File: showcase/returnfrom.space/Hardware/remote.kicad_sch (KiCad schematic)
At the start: 3 parts, among them J7 OLED, U6 ESP32-S2-SOLO

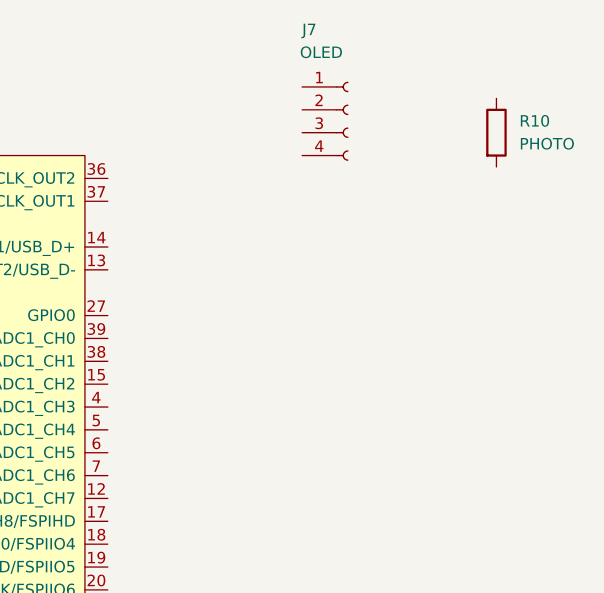
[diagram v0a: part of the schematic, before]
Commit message: updated
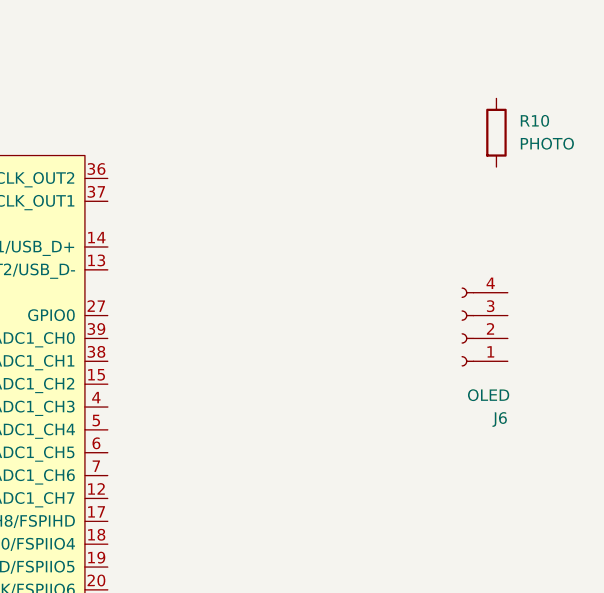
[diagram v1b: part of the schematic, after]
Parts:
- removed J7: OLED, Connector_PinSocket_2.54mm:PinSocket_1x04_P2.54mm_Vertical, symbol Connector:Conn_01x04_Socket
- added J6: OLED, TG9541:Display_128x64_096_I2C, symbol Connector:Conn_01x04_Socket
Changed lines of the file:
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@@
 	(paper "A4")
+	(symbol
+		(lib_id "Connector:Conn_01x04_Socket")
+		(at 173.99 62.23 180)
+		(unit 1)
+		(exclude_from_sim no)
+		(in_bom yes)
+		(on_board yes)
+		(dnp no)
+		(property "Reference" "J6"
+			(at 179.07 71.12 0)
+			(effects
+				(font
+					(size 1.27 1.27)
+				)
+				(justify left)
+			)
+		)
+		(property "Value" "OLED"
+			(at 179.324 68.58 0)
+			(effects
+				(font
+					(size 1.27 1.27)
+				)
+				(justify left)
+			)
+		)
+		(property "Footprint" "TG9541:Display_128x64_096_I2C"
+			(at 173.99 62.23 0)
+			(effects
+				(font
+					(size 1.27 1.27)
+				)
+				(hide yes)
+			)
+		)
+		(property "Datasheet" "~"
+			(at 173.99 62.23 0)
+			(effects
+				(font
+					(size 1.27 1.27)
+				)
+				(hide yes)
+			)
+		)
+		(property "Description" "Generic connector, single row, 01x04, script generated"
+			(at 173.99 62.23 0)
+			(effects
+				(font
+					(size 1.27 1.27)
+				)
+				(hide yes)
+			)
+		)
+		(pin "4"
+		)
+		(pin "3"
+		)
+		(pin "2"
+		)
+		(pin "1"
+		)
+		(instances
+			(project "spacescape"
+				(path "/418a52ba-b136-48f0-a485-149e9dc1363e/bd4ffa4f-b637-4be7-8de2-092b7a28716e"
+					(reference "J6")
+					(unit 1)
+				)
+			)
+		)
+	)
 	(symbol
 		(lib_id "Device:R")
@@
 					(unit 1)
 				)
-			)
-		)
-	)
-	(symbol
-		(lib_id "Connector:Conn_01x04_Socket")
-		(at 161.29 36.83 0)
-		(unit 1)
-		(exclude_from_sim no)
-		(in_bom yes)
-		(on_board yes)
-		(dnp no)
-		(property "Reference" "J7"
-			(at 156.21 27.94 0)
-			(effects
-				(font
-					(size 1.27 1.27)
-				)
-				(justify left)
-			)
-		)
-		(property "Value" "OLED"
-			(at 155.956 30.48 0)
-			(effects
-				(font
-					(size 1.27 1.27)
-				)
-				(justify left)
-			)
-		)
-		(property "Footprint" "Connector_PinSocket_2.54mm:PinSocket_1x04_P2.54mm_Vertical"
-			(at 161.29 36.83 0)
-			(effects
-				(font
-					(size 1.27 1.27)
-				)
-				(hide yes)
-			)
-		)
-		(property "Datasheet" "~"
-			(at 161.29 36.83 0)
-			(effects
-				(font
-					(size 1.27 1.27)
-				)
-				(hide yes)
-			)
-		)
-		(property "Description" "Generic connector, single row, 01x04, script generated"
-			(at 161.29 36.83 0)
-			(effects
-				(font
-					(size 1.27 1.27)
-				)
-				(hide yes)
-			)
-		)
-		(pin "4"
-		)
-		(pin "3"
-		)
-		(pin "2"
-		)
-		(pin "1"
-		)
-		(instances
-			(project "spacescape"
-				(path "/418a52ba-b136-48f0-a485-149e9dc1363e/bd4ffa4f-b637-4be7-8de2-092b7a28716e"
-					(reference "J7")
-					(unit 1)
-				)

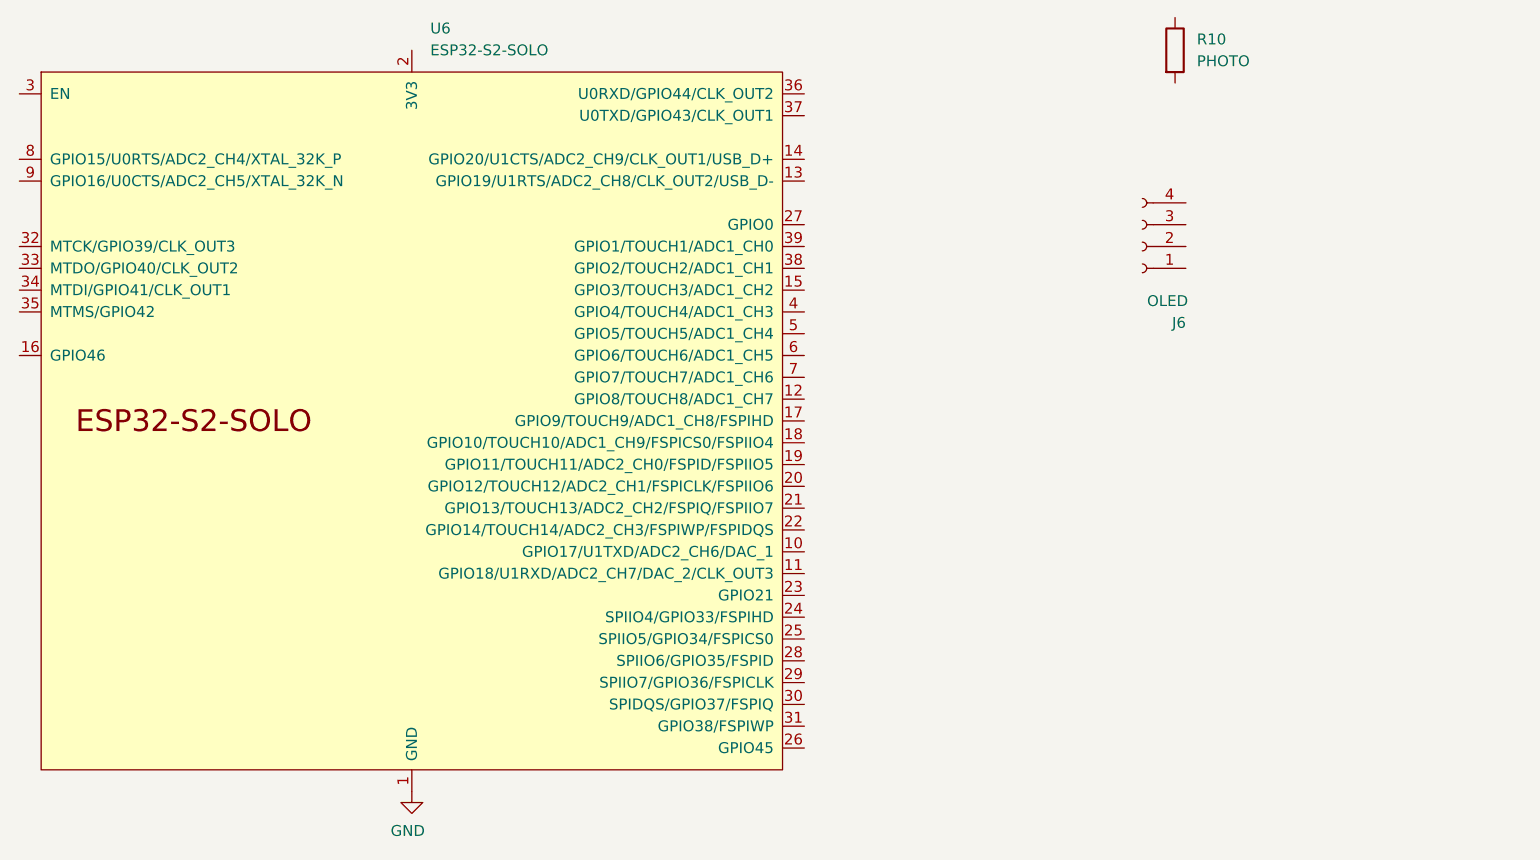
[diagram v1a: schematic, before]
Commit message: updated
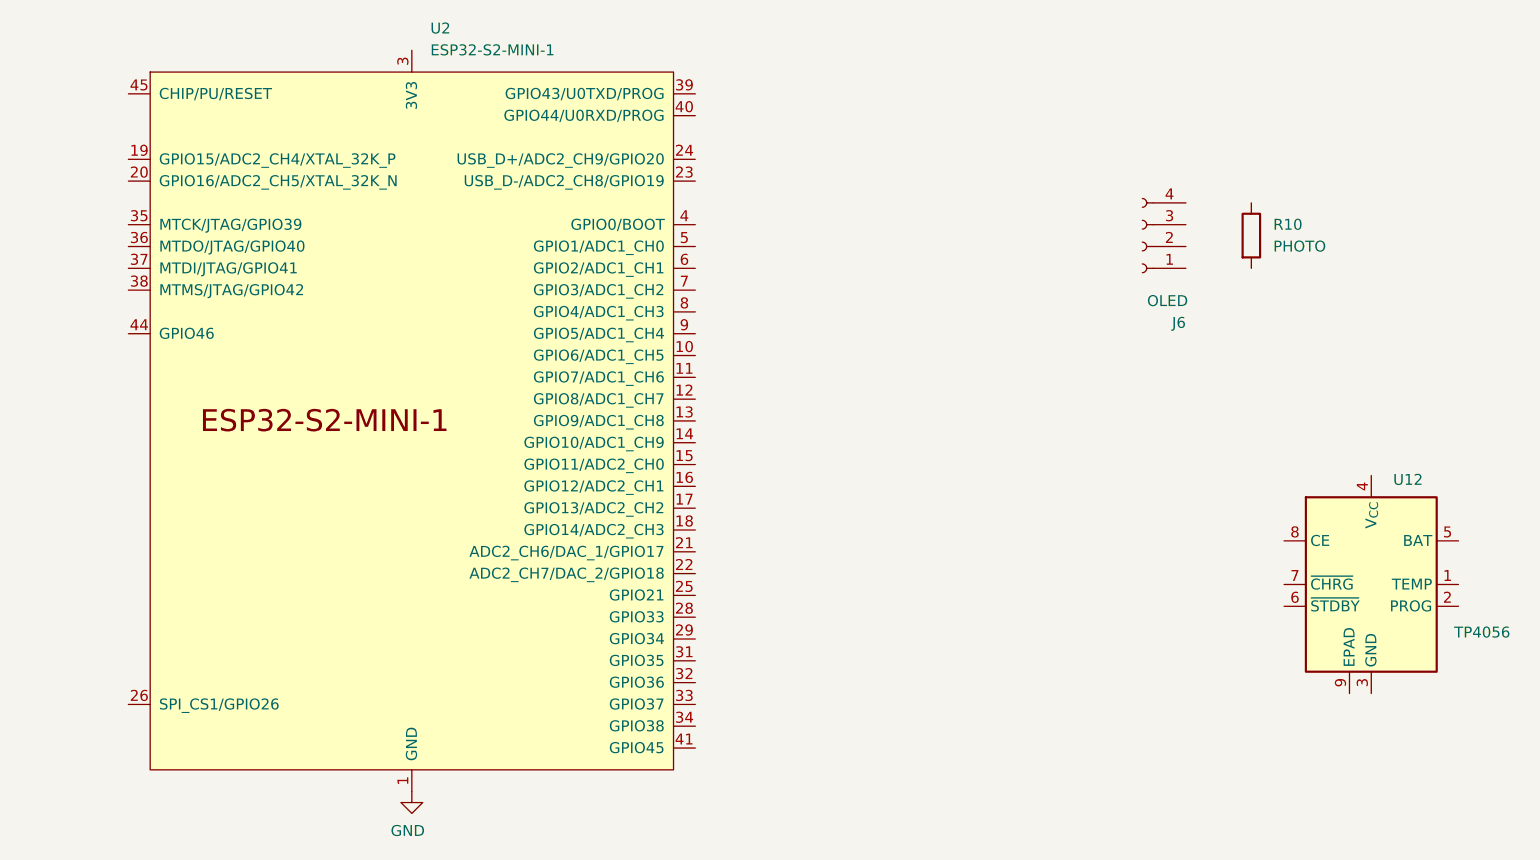
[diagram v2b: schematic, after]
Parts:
- removed U6: ESP32-S2-SOLO, Espressif:ESP32-S2-SOLO, symbol Espressif:ESP32-S2-SOLO
- added U12: TP4056, Package_SO:SOIC-8-1EP_3.9x4.9mm_P1.27mm_EP2.41x3.3mm_ThermalVias, symbol Battery_Management:TP4056-42-ESOP8
- added U2: ESP32-S2-MINI-1, Espressif:ESP32-S2-MINI-1, symbol Espressif:ESP32-S2-MINI-1
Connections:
- net GND: now also U2.1 (GND), U2.2 (GND), U2.30 (GND), U2.42 (GND), U2.43 (GND), U2.46 (GND), U2.47 (GND), U2.48 (GND), U2.49 (GND), U2.50 (GND), U2.51 (GND), U2.52 (GND), U2.53 (GND), U2.54 (GND), U2.55 (GND), U2.56 (GND), U2.57 (GND), U2.58 (GND), U2.59 (GND), U2.60 (GND), U2.61 (GND), U2.62 (GND), U2.63 (GND), U2.64 (GND), U2.65 (GND)
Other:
- moved on the sheet: R10
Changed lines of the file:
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@@
+	)
+	(symbol
+		(lib_id "Battery_Management:TP4056-42-ESOP8")
+		(at 200.66 101.6 0)
+		(unit 1)
+		(exclude_from_sim no)
+		(in_bom yes)
+		(on_board yes)
+		(dnp no)
+		(property "Reference" "U12"
+			(at 203.2 89.408 0)
+			(effects
+				(font
+					(size 1.27 1.27)
+				)
+				(justify left)
+			)
+		)
+		(property "Value" "TP4056"
+			(at 210.312 107.188 0)
+			(effects
+				(font
+					(size 1.27 1.27)
+				)
+				(justify left)
+			)
+		)
+		(property "Footprint" "Package_SO:SOIC-8-1EP_3.9x4.9mm_P1.27mm_EP2.41x3.3mm_ThermalVias"
+			(at 201.168 124.46 0)
+			(effects
+				(font
+					(size 1.27 1.27)
+				)
+				(hide yes)
+			)
+		)
+		(property "Datasheet" "C22451416"
+			(at 200.66 127 0)
+			(effects
+				(font
+					(size 1.27 1.27)
+				)
+				(hide yes)
+			)
+		)
+		(property "Description" "1A Standalone Linear Li-ion/LiPo single-cell battery charger, 4.2V ±1% charge voltage, VCC = 4.0..8.0V, SOIC-8 (SOP-8)"
+			(at 201.168 121.92 0)
+			(effects
+				(font
+					(size 1.27 1.27)
+				)
+				(hide yes)
+			)
+		)
+		(pin "6"
+		)
+		(pin "8"
+		)
+		(pin "7"
+		)
+		(pin "4"
+		)
+		(pin "9"
+		)
+		(pin "1"
+		)
+		(pin "5"
+		)
+		(pin "2"
+		)
+		(pin "3"
+		)
+		(instances
+			(project "spacescape"
+				(path "/418a52ba-b136-48f0-a485-149e9dc1363e/bd4ffa4f-b637-4be7-8de2-092b7a28716e"
+					(reference "U12")
+					(unit 1)
+				)
+			)
+		)
 	)
 	(symbol
 		(lib_id "Device:R")
-		(at 177.8 39.37 0)
+		(at 186.69 60.96 0)
 		(unit 1)
 		(exclude_from_sim no)
@@
 		(fields_autoplaced yes)
 		(property "Reference" "R10"
-			(at 180.34 38.0999 0)
+			(at 189.23 59.6899 0)
 			(effects
 				(font
@@
 		)
 		(property "Value" "PHOTO"
-			(at 180.34 40.6399 0)
+			(at 189.23 62.2299 0)
 			(effects
 				(font
@@
 		)
 		(property "Footprint" "Resistor_SMD:R_1210_3225Metric"
-			(at 176.022 39.37 90)
+			(at 184.912 60.96 90)
 			(effects
 				(font
@@
 		)
 		(property "Datasheet" "C2904883"
-			(at 177.8 39.37 0)
+			(at 186.69 60.96 0)
 			(effects
 				(font
@@
 		)
 		(property "Description" "Resistor"
-			(at 177.8 39.37 0)
+			(at 186.69 60.96 0)
 			(effects
 				(font
@@
 	)
 	(symbol
-		(lib_id "Espressif:ESP32-S2-SOLO")
+		(lib_id "Espressif:ESP32-S2-MINI-1")
 		(at 88.9 82.55 0)
 		(unit 1)
@@
 		(dnp no)
 		(fields_autoplaced yes)
-		(property "Reference" "U6"
+		(property "Reference" "U2"
 			(at 91.0433 36.83 0)
 			(effects
@@
 			)
 		)
-		(property "Value" "ESP32-S2-SOLO"
+		(property "Value" "ESP32-S2-MINI-1"
 			(at 91.0433 39.37 0)
 			(effects
@@
 			)
 		)
-		(property "Footprint" "Espressif:ESP32-S2-SOLO"
+		(property "Footprint" "Espressif:ESP32-S2-MINI-1"
 			(at 88.9 135.89 0)
 			(effects
@@
 			)
 		)
-		(property "Datasheet" "https://www.espressif.com/sites/default/files/documentation/esp32-s2-solo_esp32-s2-solo-u_datasheet_en.pdf"
-			(at 88.9 138.43 0)
-			(effects
-				(font
-					(size 1.27 1.27)
-				)
-				(hide yes)
-			)
-		)
-		(property "Description" "ESP32-S2-SOLO and ESP32-S2-SOLO-U are two powerful, generic Wi-Fi MCU modules that have a rich set of peripherals."
+		(property "Datasheet" "https://www.espressif.com/sites/default/files/documentation/esp32-s2-mini-1_esp32-s2-mini-1u_datasheet_en.pdf"
+			(at 91.44 138.43 0)
+			(effects
+				(font
+					(size 1.27 1.27)
+				)
+				(hide yes)
+			)
+		)
+		(property "Description" "ESP32-S2-MINI-1 and ESP32-S2-MINI-1U are two powerful, generic Wi-Fi MCU modules that have a rich set of peripherals. They are an ideal choice for a wide variety of application scenarios relating to Internet of Things (IoT), wearable electronics and smart home."
 			(at 88.9 82.55 0)
 			(effects
@@
 			)
 		)
+		(pin "10"
+		)
+		(pin "15"
+		)
+		(pin "18"
+		)
+		(pin "6"
+		)
+		(pin "25"
+		)
+		(pin "9"
+		)
+		(pin "11"
+		)
+		(pin "13"
+		)
+		(pin "16"
+		)
 		(pin "4"
 		)
@@
 		(pin "8"
 		)
+		(pin "12"
+		)
+		(pin "5"
+		)
+		(pin "14"
+		)
+		(pin "17"
+		)
+		(pin "22"
+		)
+		(pin "21"
+		)
+		(pin "28"
+		)
+		(pin "29"
+		)
+		(pin "31"
+		)
 		(pin "32"
 		)
+		(pin "33"
+		)
+		(pin "34"
+		)
 		(pin "41"
 		)
-		(pin "9"
-		)
-		(pin "34"
+		(pin "46"
+		)
+		(pin "54"
+		)
+		(pin "63"
+		)
+		(pin "49"
+		)
+		(pin "58"
+		)
+		(pin "35"
+		)
+		(pin "36"
+		)
+		(pin "26"
+		)
+		(pin "44"
+		)
+		(pin "48"
+		)
+		(pin "61"
+		)
+		(pin "65"
+		)
+		(pin "1"
+		)
+		(pin "55"
+		)
+		(pin "45"
+		)
+		(pin "47"
+		)
+		(pin "43"
+		)
+		(pin "51"
+		)
+		(pin "52"
+		)
+		(pin "50"
+		)
+		(pin "57"
+		)
+		(pin "59"
+		)
+		(pin "53"
+		)
+		(pin "56"
+		)
+		(pin "60"
+		)
+		(pin "62"
+		)
+		(pin "64"
+		)
+		(pin "19"
+		)
+		(pin "20"
+		)
+		(pin "37"
+		)
+		(pin "38"
+		)
+		(pin "24"
+		)
+		(pin "23"
+		)
+		(pin "27"
+		)
+		(pin "3"
 		)
 		(pin "2"
 		)
-		(pin "1"
-		)
-		(pin "14"
-		)
-		(pin "13"
-		)
-		(pin "35"
-		)
-		(pin "3"
-		)
-		(pin "16"
+		(pin "30"
+		)
+		(pin "42"
 		)
 		(pin "39"
 		)
-		(pin "38"
-		)
-		(pin "33"
-		)
-		(pin "15"
-		)
-		(pin "36"
-		)
 		(pin "40"
 		)
-		(pin "37"
-		)
-		(pin "27"
-		)
-		(pin "5"
-		)
-		(pin "6"
-		)
-		(pin "12"
-		)
-		(pin "17"
-		)
-		(pin "18"
-		)
-		(pin "19"
-		)
-		(pin "31"
-		)
-		(pin "10"
-		)
-		(pin "28"
-		)
-		(pin "21"
-		)
-		(pin "11"
-		)
-		(pin "26"
-		)
-		(pin "20"
-		)
-		(pin "23"
-		)
-		(pin "30"
-		)
-		(pin "25"
-		)
-		(pin "29"
-		)
-		(pin "24"
-		)
-		(pin "22"
-		)
 		(instances
-			(project "spacescape"
+			(project ""
 				(path "/418a52ba-b136-48f0-a485-149e9dc1363e/bd4ffa4f-b637-4be7-8de2-092b7a28716e"
-					(reference "U6")
+					(reference "U2")
 					(unit 1)
 				)
